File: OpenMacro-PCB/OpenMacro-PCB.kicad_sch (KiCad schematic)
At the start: 16 parts, among them P1 RFID-RC522-MODULE, SW1 SW_Push, SW2 SW_Push, SW3 SW_Push, SW4 SW_Push, SW5 SW_Push, SW6 SW_Push, SW7 SW_Push, SW8 SW_Push, SW9 SW_Push, U1 AMS1117-3.3, U2 Arduino_Micro

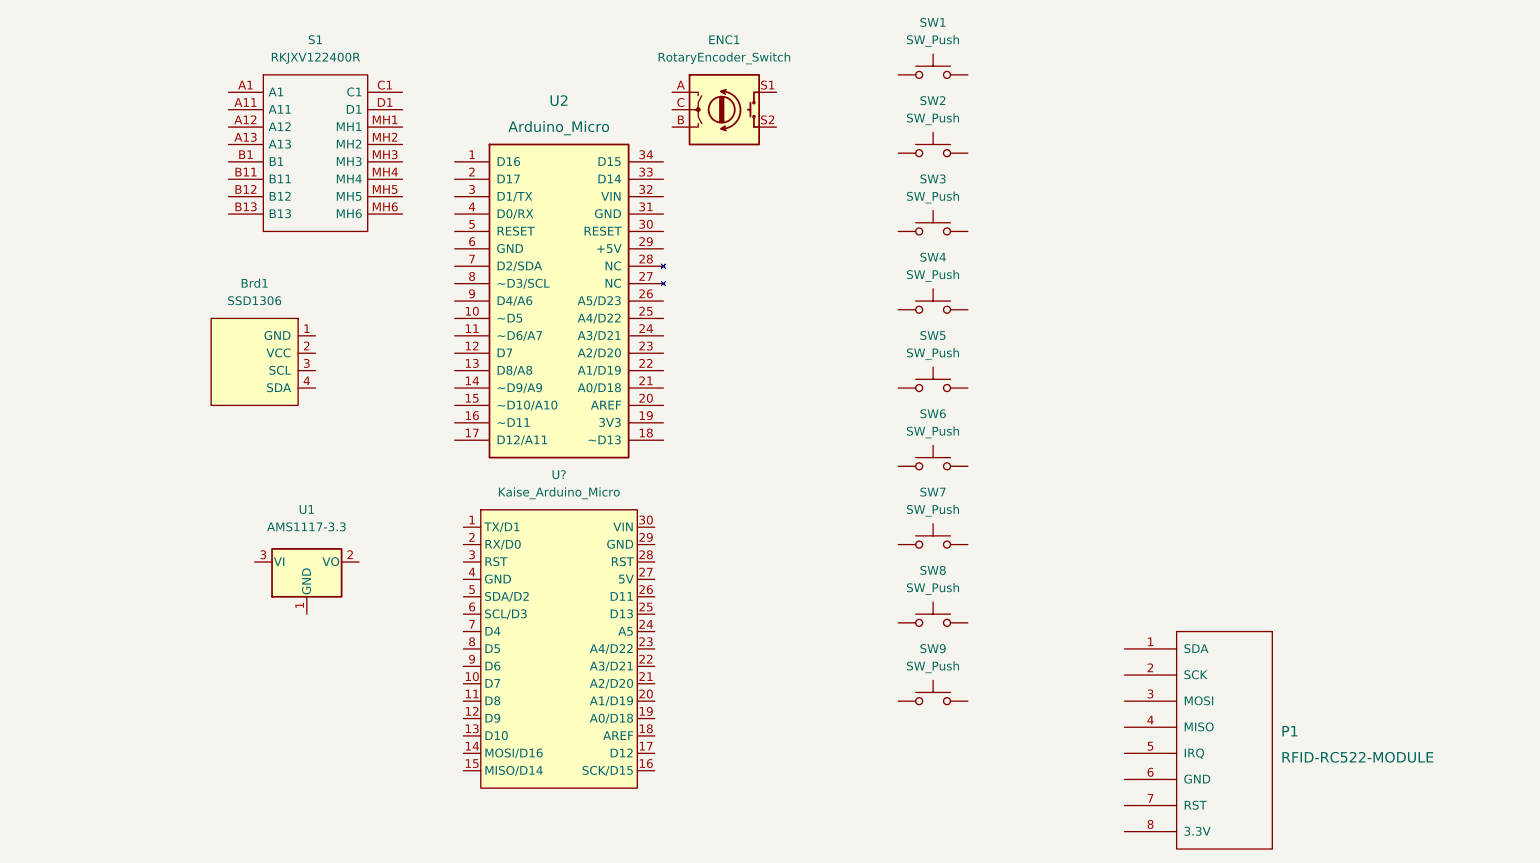
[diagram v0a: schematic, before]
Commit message: Update kicad_sch.
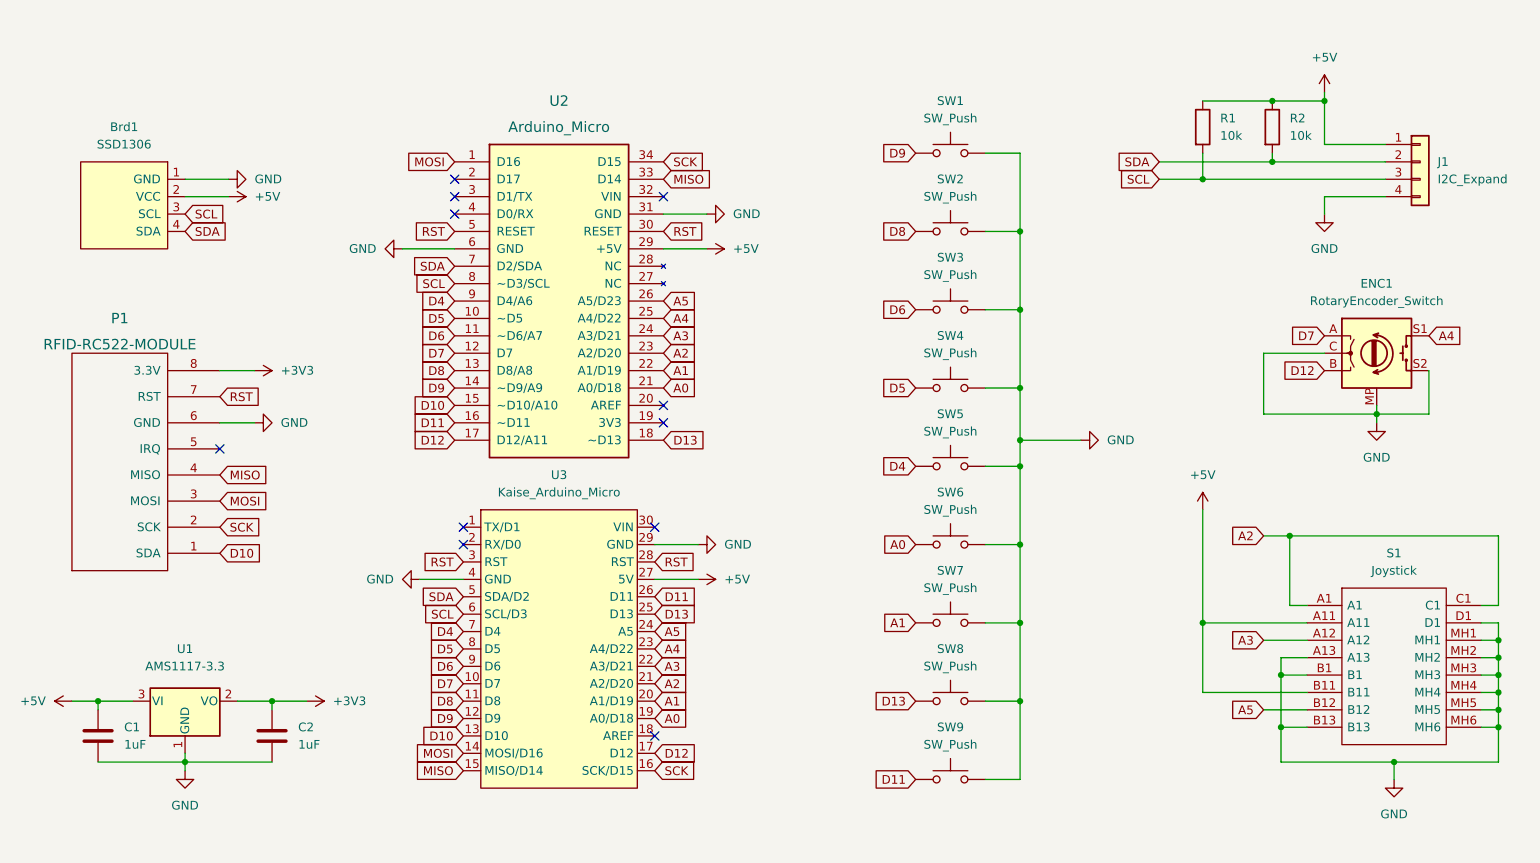
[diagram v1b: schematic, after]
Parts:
- added C1, C2: 1uF, Capacitor_SMD:C_1206_3216Metric_Pad1.33x1.80mm_HandSolder, symbol Device:C
- added J1: I2C_Expand, Connector_PinSocket_2.54mm:PinSocket_1x04_P2.54mm_Horizontal, symbol Connector_Generic:Conn_01x04
- added R1, R2: 10k, Resistor_SMD:R_1206_3216Metric_Pad1.30x1.75mm_HandSolder, symbol Device:R
- ENC1: footprint Rotary_Encoder:RotaryEncoder_Alps_EC11E-Switch_Vertical_H20mm -> Rotary_Encoder:RotaryEncoder_Alps_EC11E-Switch_Vertical_H20mm_CircularMountingHoles
- S1: value RKJXV122400R -> Joystick
- U3: renamed from U?; footprint (none) -> Audio_Module:Kaise_Arduino_Micro
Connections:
- net D7: now reaches U3.10 (D7)
- net D7: now also ENC1.A, U2.12 (D7)
- net D8: now reaches U3.11 (D8)
- net D8: now also SW2.1, U2.13 (D8/A8)
- net D9: now reaches U3.12 (D9)
- net D9: now also SW1.1, U2.14 (~D9/A9)
- net D10: now reaches U3.13 (D10)
- net D10: now also P1.1 (SDA), U2.15 (~D10/A10)
- net MOSI: now reaches U3.14 (MOSI/D16)
- net MOSI: now also P1.3 (MOSI), U2.1 (D16)
- net MISO: now reaches U3.15 (MISO/D14)
- net MISO: now also P1.4 (MISO), U2.33 (D14)
- net SCK: now reaches U3.16 (SCK/D15)
- net SCK: now also P1.2 (SCK), U2.34 (D15)
- net D12: now reaches U3.17 (D12)
- net D12: now also ENC1.B, U2.17 (D12/A11)
- net A0: now reaches U3.19 (A0/D18)
- net A0: now also SW6.1, U2.21 (A0/D18)
- net A1: now reaches U3.20 (A1/D19)
- net A1: now also SW7.1, U2.22 (A1/D19)
- net A2: now reaches U3.21 (A2/D20)
- net A2: now also S1.A1, S1.C1, U2.23 (A2/D20)
- net A3: now reaches U3.22 (A3/D21)
- net A3: now also S1.A12, U2.24 (A3/D21)
- net A4: now reaches U3.23 (A4/D22)
- net A4: now also ENC1.S1, U2.25 (A4/D22)
- net A5: now reaches U3.24 (A5)
- net A5: now also S1.B12, U2.26 (A5/D23)
- net D13: now reaches U3.25 (D13)
- net D13: now also SW8.1, U2.18 (~D13)
- net D11: now reaches U3.26 (D11)
- net D11: now also SW9.1, U2.16 (~D11)
- net +5V: now reaches U3.27 (5V)
- net +5V: now also Brd1.2 (VCC), S1.A11, S1.B11, U1.3 (VI), U2.29 (+5V), C1.1, J1.1 (Pin_1), R1.1, R2.1
- net RST: now reaches U3.28 (RST)
- net RST: now also P1.7 (RST), U2.30 (RESET), U2.5 (RESET), U3.3 (RST)
- net GND: now reaches U3.29 (GND)
- net GND: now also Brd1.1 (GND), ENC1.C, ENC1.MP, ENC1.S2, P1.6 (GND), S1.A13, S1.B1, S1.B13, S1.D1, S1.MH1, S1.MH2, S1.MH3, S1.MH4, S1.MH5, S1.MH6, SW1.2, SW2.2, SW3.2, SW4.2, SW5.2, SW6.2, SW7.2, SW8.2, SW9.2, U1.1 (GND), U2.31 (GND), U2.6 (GND), U3.4 (GND), C1.2, C2.2, J1.4 (Pin_4)
- net SDA: now reaches U3.5 (SDA/D2)
- net SDA: now also Brd1.4 (SDA), U2.7 (D2/SDA), J1.2 (Pin_2), R2.2
- net SCL: now reaches U3.6 (SCL/D3)
- net SCL: now also Brd1.3 (SCL), U2.8 (~D3/SCL), J1.3 (Pin_3), R1.2
- net D4: now reaches U3.7 (D4)
- net D4: now also SW5.1, U2.9 (D4/A6)
- net D5: now reaches U3.8 (D5)
- net D5: now also SW4.1, U2.10 (~D5)
- net D6: now reaches U3.9 (D6)
- net D6: now also SW3.1, U2.11 (~D6/A7)
- net +3V3: now reaches U1.2 (VO)
- net +3V3: now also P1.8 (3.3V), C2.1
- no-connect marks 0 -> 11
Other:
- moved on the sheet: Brd1, P1, S1, SW1, SW2, SW3, SW4, SW5, SW6, SW7, SW8, SW9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
